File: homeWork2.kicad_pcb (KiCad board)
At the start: 2 copper layers, 125 x 99.9 mm, 43 parts, among them J1 Barrel_Jack_Switch_SMT, U1 LM7805_TO220

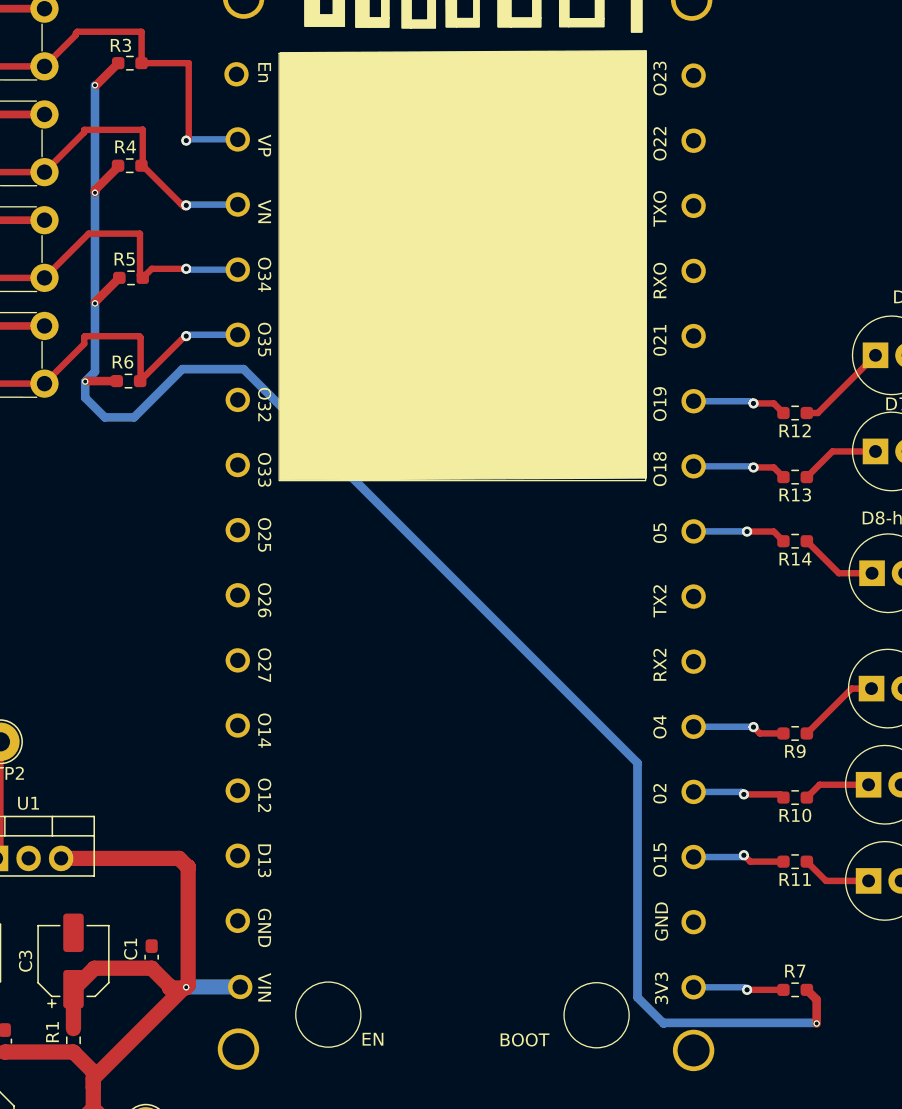
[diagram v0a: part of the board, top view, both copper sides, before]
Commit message: Gerber files and enhancements file are added,
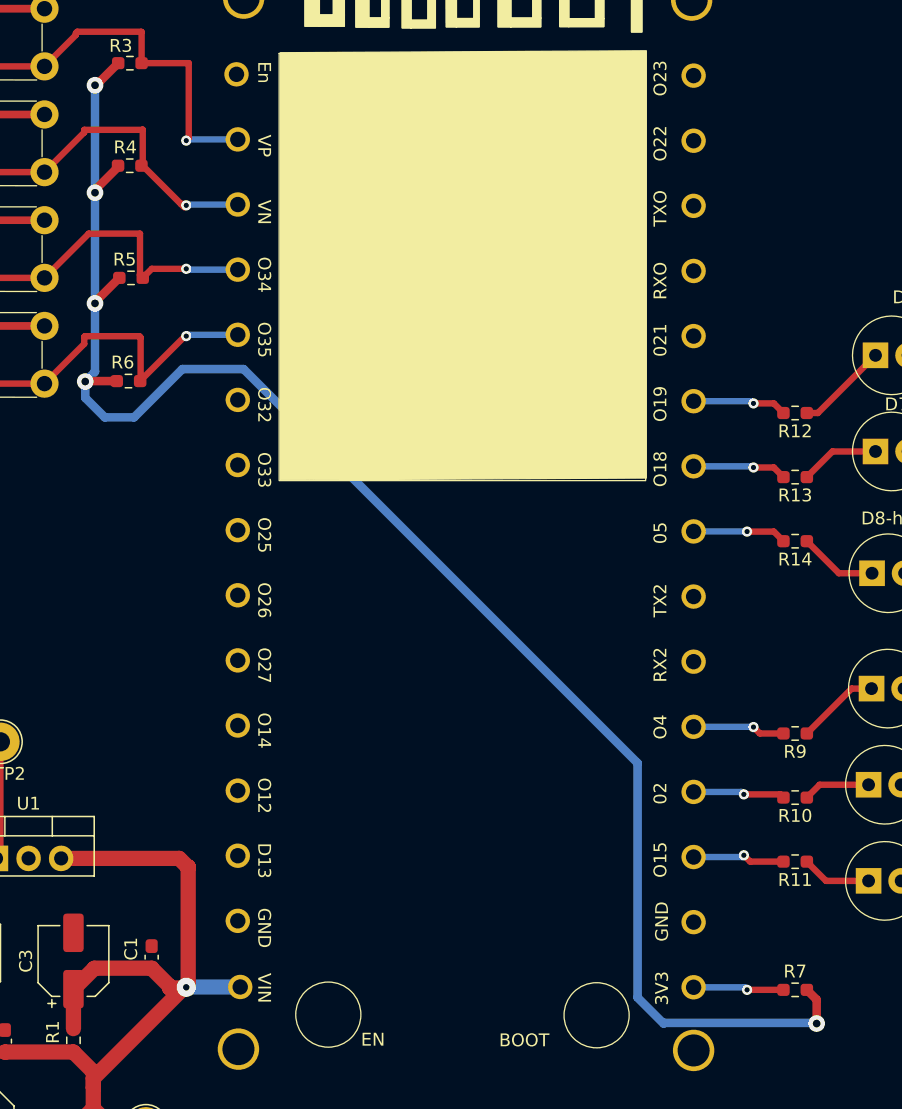
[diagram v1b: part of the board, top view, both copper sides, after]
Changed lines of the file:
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@@
     (pts (xy 50 150) (xy 170 150))
     (height 10)
-    (gr_text "120.0000 mm" (at 110 158.85) (layer "Dwgs.User")
+    (gr_text "4724.4094 mils" (at 110 158.85) (layer "Dwgs.User")
       (effects (font (size 1 1) (thickness 0.15)))
     )
@@
     (pts (xy 175 50) (xy 50 50))
     (height 10)
-    (gr_text "125.0000 mm" (at 112.5 38.85) (layer "Dwgs.User")
+    (gr_text "4921.2598 mils" (at 112.5 38.85) (layer "Dwgs.User")
       (effects (font (size 1 1) (thickness 0.15)))
     )
@@
     (pts (xy 50 150) (xy 50 128))
     (height -7)
-    (gr_text "22.0000 mm" (at 41.85 139 90) (layer "Dwgs.User")
+    (gr_text "866.1417 mils" (at 41.85 139 90) (layer "Dwgs.User")
       (effects (font (size 1 1) (thickness 0.15)))
     )
@@
     (pts (xy 50 50) (xy 50 150))
     (height 11)
-    (gr_text "100.0000 mm" (at 37.85 100 90) (layer "Dwgs.User")
+    (gr_text "3937.0079 mils" (at 37.85 100 90) (layer "Dwgs.User")
       (effects (font (size 1 1) (thickness 0.15)))
     )
@@
     (pts (xy 50 150) (xy 50 55))
     (height -9)
-    (gr_text "95.0000 mm" (at 39.85 102.5 90) (layer "Dwgs.User")
+    (gr_text "3740.1575 mils" (at 39.85 102.5 90) (layer "Dwgs.User")
       (effects (font (size 1 1) (thickness 0.15)))
     )
@@
     (pts (xy 50 150) (xy 50 145))
     (height -4)
-    (gr_text "5.0000 mm" (at 44.85 147.5 90) (layer "Dwgs.User")
+    (gr_text "196.8504 mils" (at 44.85 147.5 90) (layer "Dwgs.User")
       (effects (font (size 1 1) (thickness 0.15)))
     )
@@
     (pts (xy 47 128) (xy 50 128))
     (height 14)
-    (gr_text "3.0000 mm" (at 48.5 140.85) (layer "Dwgs.User")
+    (gr_text "118.1102 mils" (at 48.5 140.85) (layer "Dwgs.User")
       (effects (font (size 1 1) (thickness 0.15)))
     )
@@
   (segment (start 97.75 140.15) (end 97.75 138.9) (width 1.19) (layer "F.Cu") (net 3))
   (segment (start 103.7 132.2125) (end 103.7 132.35) (width 1.19) (layer "F.Cu") (net 3))
-  (segment (start 97.75 139.4) (end 97.75 140.15) (width 1.19) (layer "F.Cu") (net 3))
   (segment (start 91 143.25) (end 92.9125 143.25) (width 1.19) (layer "F.Cu") (net 3))
   (segment (start 96.2 137.35) (end 90.8625 137.35) (width 1.19) (layer "F.Cu") (net 3))
@@
   (segment (start 105.1 122.9) (end 105.15 122.9) (width 1.19) (layer "F.Cu") (net 3))
   (segment (start 97.75 138.9) (end 96.2 137.35) (width 1.19) (layer "F.Cu") (net 3))
+  (segment (start 104.85 132.3) (end 97.75 139.4) (width 1.19) (layer "F.Cu") (net 3))
   (segment (start 94.5 144.8375) (end 94.6625 144.8375) (width 1.19) (layer "F.Cu") (net 3))
+  (segment (start 105 132.3) (end 104.85 132.3) (width 1.19) (layer "F.Cu") (net 3))
   (segment (start 105.15 122.9) (end 105.15 122.95) (width 1.19) (layer "F.Cu") (net 3))
   (segment (start 95.24 122.245) (end 104.445 122.245) (width 1.19) (layer "F.Cu") (net 3))
+  (segment (start 105 132.3) (end 104.95 132.35) (width 1.19) (layer "F.Cu") (net 3))
+  (segment (start 105 132.3) (end 105.15 132.15) (width 1.19) (layer "F.Cu") (net 3))
   (segment (start 105.15 122.95) (end 105.05 122.85) (width 1.19) (layer "F.Cu") (net 3))
   (segment (start 97.75 141.75) (end 99.15 143.15) (width 1.19) (layer "F.Cu") (net 3))
@@
   (segment (start 103.7 132.35) (end 103.8375 132.35) (width 1.19) (layer "F.Cu") (net 3))
   (segment (start 104.445 122.245) (end 105.1 122.9) (width 1.19) (layer "F.Cu") (net 3))
-  (segment (start 105 132.3) (end 104.95 132.35) (width 1.19) (layer "F.Cu") (net 3))
-  (segment (start 104.85 132.3) (end 97.75 139.4) (width 1.19) (layer "F.Cu") (net 3))
   (segment (start 97.8375 130.8125) (end 96.2 132.45) (width 1.19) (layer "F.Cu") (net 3))
+  (segment (start 97.75 139.4) (end 97.75 140.15) (width 1.19) (layer "F.Cu") (net 3))
   (segment (start 104.95 132.35) (end 103.7 132.35) (width 1.19) (layer "F.Cu") (net 3))
-  (segment (start 105 132.3) (end 105.15 132.15) (width 1.19) (layer "F.Cu") (net 3))
   (segment (start 97.75 141.75) (end 97.75 140.15) (width 1.19) (layer "F.Cu") (net 3))
   (segment (start 96.2 132.45) (end 96.2 135.525) (width 1.19) (layer "F.Cu") (net 3))
   (segment (start 99.15 143.15) (end 101.85 143.15) (width 1.19) (layer "F.Cu") (net 3))
-  (segment (start 105 132.3) (end 104.85 132.3) (width 1.19) (layer "F.Cu") (net 3))
   (segment (start 105.15 132.15) (end 105.15 122.95) (width 1.19) (layer "F.Cu") (net 3))
-  (via (at 105 132.3) (size 0.5) (drill 0.3) (layers "F.Cu" "B.Cu") (net 3))
-  (segment (start 105.023 132.277) (end 105 132.3) (width 1.19) (layer "B.Cu") (net 3))
-  (segment (start 109.2107 132.277) (end 105.023 132.277) (width 1.19) (layer "B.Cu") (net 3))
+  (via (at 105 132.3) (size 1.5) (drill 0.5) (layers "F.Cu" "B.Cu") (net 3))
+  (segment (start 105.023 132.277) (end 109.2107 132.277) (width 1.19) (layer "B.Cu") (net 3))
+  (segment (start 105 132.3) (end 105.023 132.277) (width 1.19) (layer "B.Cu") (net 3))
   (segment (start 82.5 119.2) (end 82.5 116.925) (width 0.5) (layer "F.Cu") (net 5))
   (segment (start 82.5 116.925) (end 83.075 116.35) (width 0.5) (layer "F.Cu") (net 5))
@@
   (segment (start 99.679 68.308) (end 97.8815 70.1055) (width 0.67) (layer "F.Cu") (net 21))
   (segment (start 99.579 85.008) (end 97.1915 85.008) (width 0.67) (layer "F.Cu") (net 21))
-  (via (at 97.8815 70.312) (size 0.5) (drill 0.3) (layers "F.Cu" "B.Cu") (net 21))
-  (via (at 97.8815 61.93) (size 0.5) (drill 0.3) (layers "F.Cu" "B.Cu") (net 21))
-  (via (at 97.1195 85.044) (size 0.5) (drill 0.3) (layers "F.Cu" "B.Cu") (net 21))
-  (via (at 154.178 135.128) (size 0.5) (drill 0.3) (layers "F.Cu" "B.Cu") (net 21))
-  (via (at 97.8815 78.948) (size 0.5) (drill 0.3) (layers "F.Cu" "B.Cu") (net 21))
+  (via (at 97.8815 70.312) (size 1.3) (drill 0.6) (layers "F.Cu" "B.Cu") (net 21))
+  (via (at 97.8815 61.93) (size 1.3) (drill 0.6) (layers "F.Cu" "B.Cu") (net 21))
+  (via (at 97.1195 85.044) (size 1.3) (drill 0.6) (layers "F.Cu" "B.Cu") (net 21))
+  (via (at 154.178 135.128) (size 1.3) (drill 0.6) (layers "F.Cu" "B.Cu") (net 21))
+  (via (at 97.8815 78.948) (size 1.3) (drill 0.6) (layers "F.Cu" "B.Cu") (net 21))
   (segment (start 142.24 135.128) (end 142.291249 135.076751) (width 0.67) (layer "B.Cu") (net 21))
   (segment (start 97.1195 86.314) (end 98.6435 87.838) (width 0.67) (layer "B.Cu") (net 21))

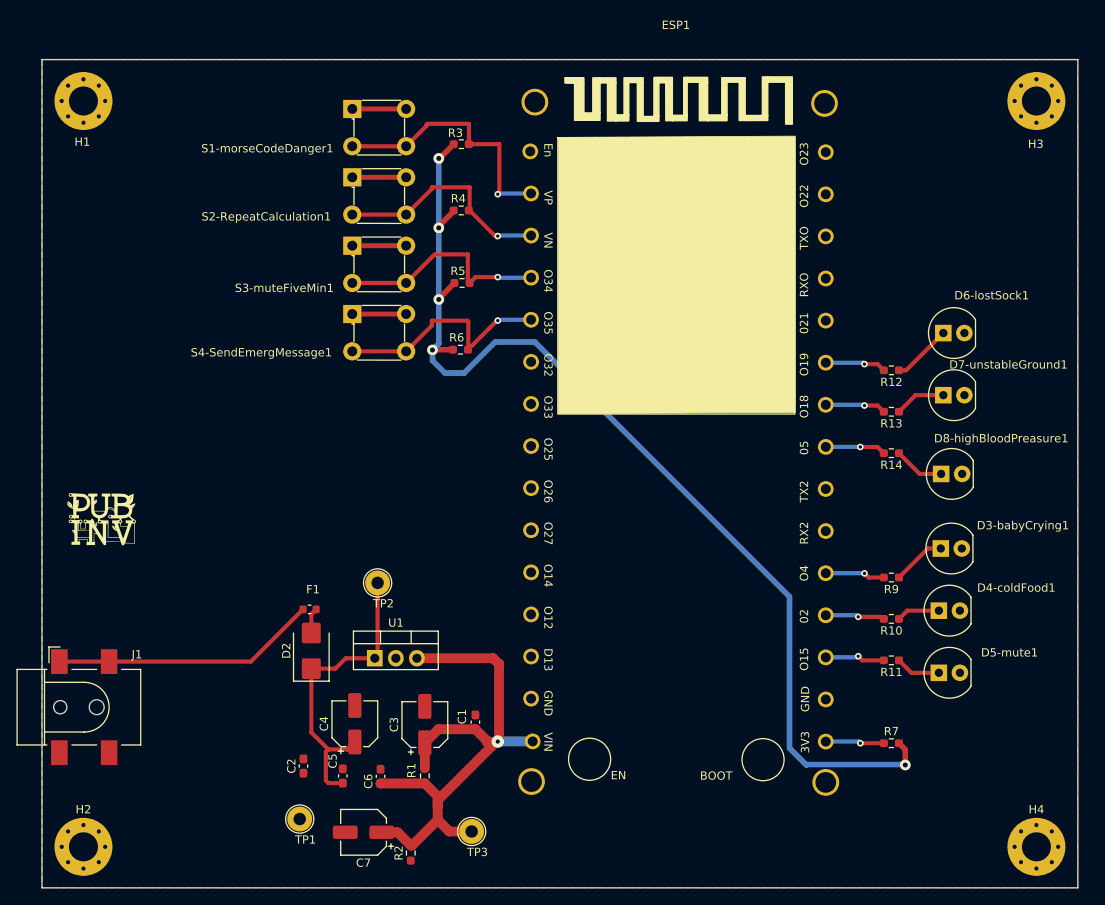
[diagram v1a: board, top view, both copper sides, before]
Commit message: updates to the pcb and the schematics.
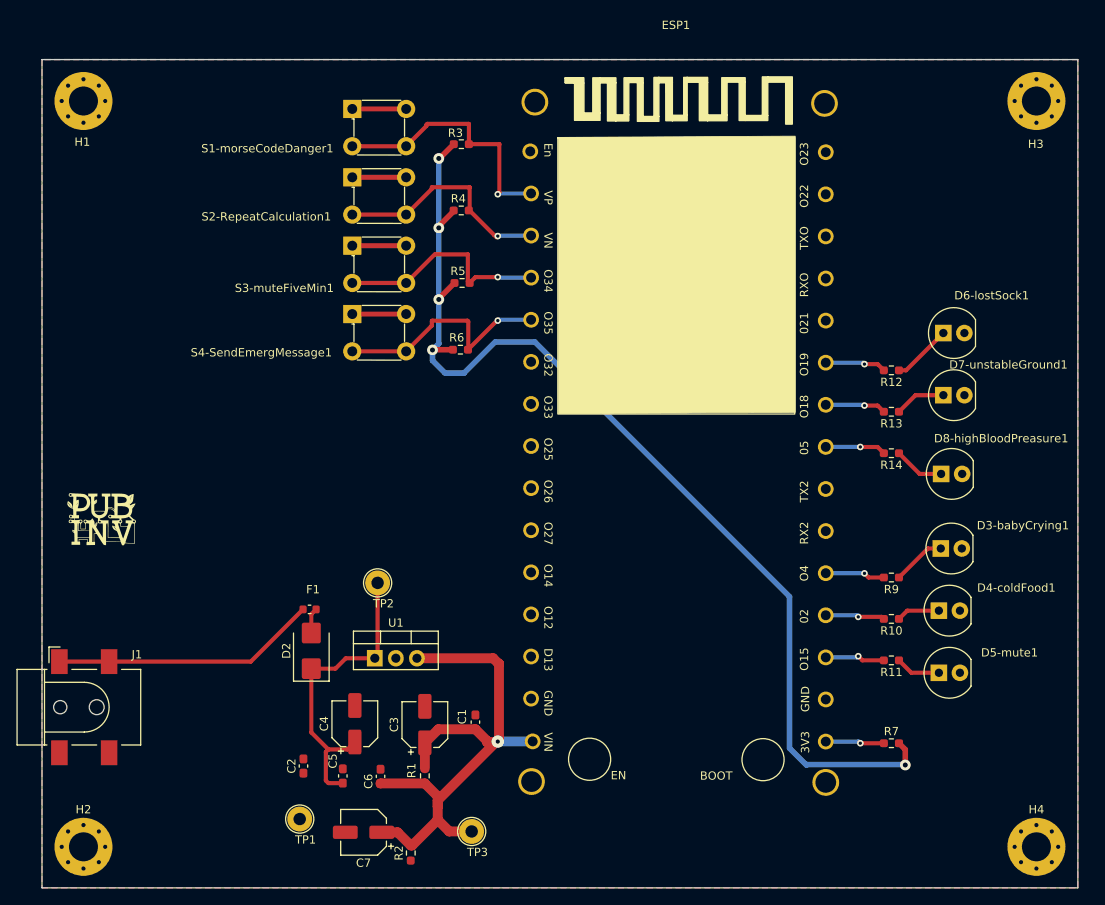
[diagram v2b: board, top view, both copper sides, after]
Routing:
- added copper zone on B.Cu, net GND
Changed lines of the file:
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@@
+    )
+  )
+  (zone (net 1) (net_name "GND") (layer "B.Cu") (hatch edge 0.5)
+    (connect_pads thru_hole_only (clearance 0))
+    (min_thickness 0.25) (filled_areas_thickness no)
+    (fill yes (thermal_gap 0.5) (thermal_bridge_width 0.5))
+    (polygon
+      (pts
+        (xy 175 50)
+        (xy 50.05 50)
+        (xy 50 50.05)
+        (xy 50 149.95)
+        (xy 174.95 149.95)
+        (xy 175 149.9)
+      )
     )
   )
